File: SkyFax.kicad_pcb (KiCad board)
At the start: 2 copper layers, 50.9 x 101.5 mm, 80 parts, among them J1 RJ11/12, J2 USB_B_Micro, J3 Conn_02x06_Odd_Even, J4 Conn_02x02_Odd_Even, Q1 Q_NPN_BEC, Q2 Q_PNP_BEC, Q3 Q_NPN_BEC, Q4 Q_NPN_BEC, Q5 Q_NPN_BEC, Q6 Q_NPN_EBC, SW2 SW_Push, U1 Si2494-A-FM, U2 Si3018, U3 25LC640AT-E/SN, U4 CP2102N-Axx-xQFN20, X1 ECS-2520MV-xxx-xx

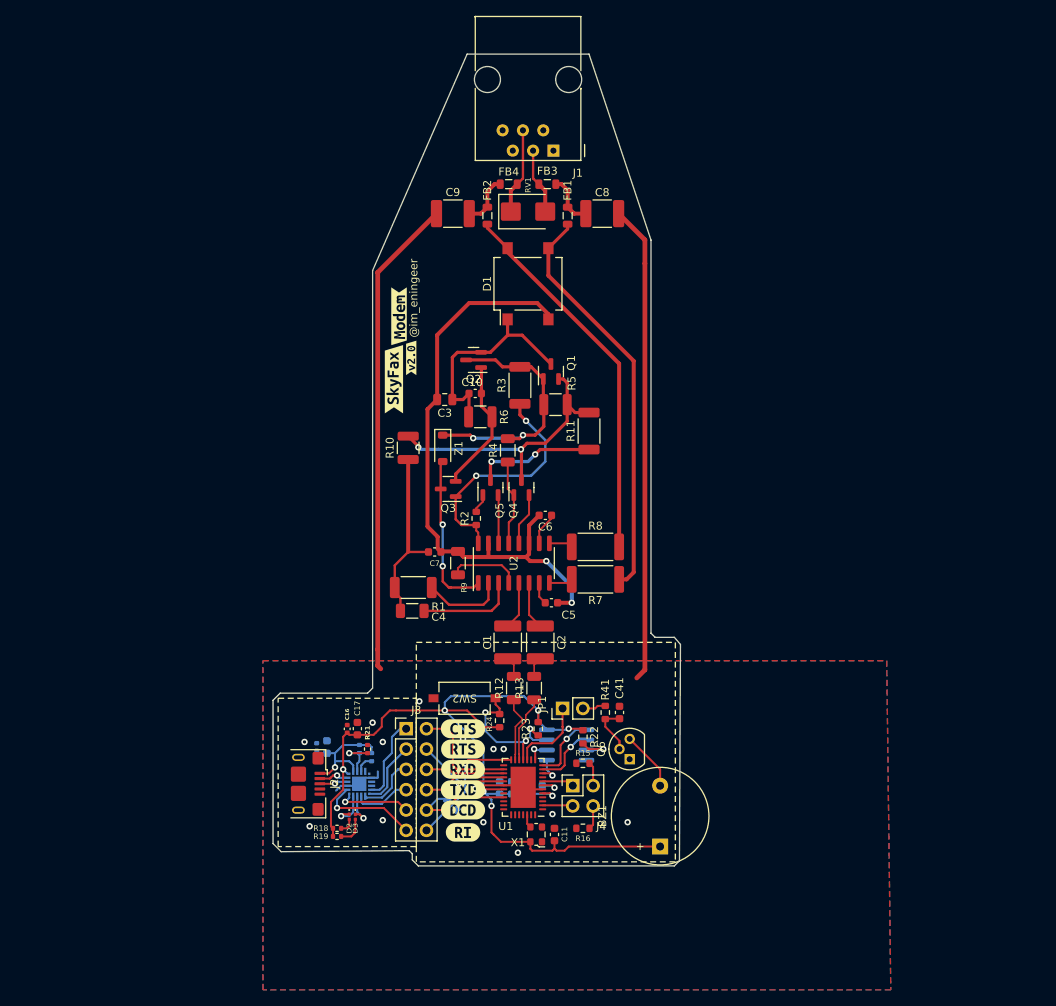
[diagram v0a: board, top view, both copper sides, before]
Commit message: Sent to fab v3.0
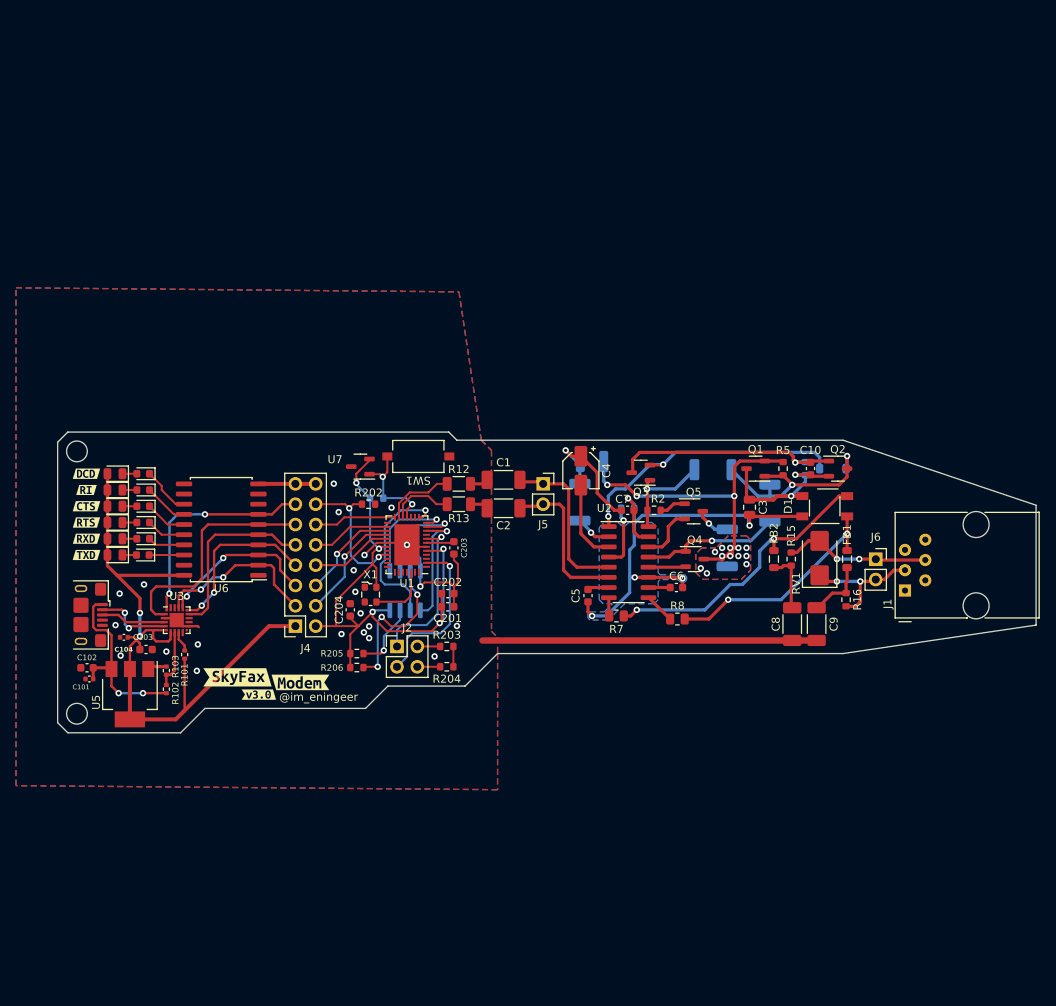
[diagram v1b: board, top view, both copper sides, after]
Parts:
- removed BZ1: Buzzer, Buzzer_Beeper:Buzzer_12x9.5RM7.6
- removed C11, C12, C17, C41, C50, C52: 0.1uF, Capacitor_SMD:C_0603_1608Metric
- removed C13, C16: 4.7uF, Capacitor_SMD:C_0402_1005Metric
- removed C51: 0.22uF, Capacitor_SMD:C_0603_1608Metric
- removed FB3, FB4: FerriteBead_Small, Inductor_SMD:L_0805_2012Metric
- removed JP1: Jumper_2_Open, Connector_PinHeader_2.54mm:PinHeader_1x02_P2.54mm_Vertical
- removed Q6: Q_NPN_EBC, Package_TO_SOT_THT:TO-92
- removed R14, R22, R23, R24: 10k, Resistor_SMD:R_0603_1608Metric
- removed R17: 1k, Resistor_SMD:R_0402_1005Metric
- removed R18, R19: 220, Resistor_SMD:R_0402_1005Metric
- removed R20: 22.1k, Resistor_SMD:R_0402_1005Metric
- removed R21: 47.5k, Resistor_SMD:R_0402_1005Metric
- removed R41: 150, Resistor_SMD:R_0603_1608Metric
- removed SW2: SW_Push, Button_Switch_SMD:SW_Tactile_SPST_NO_Straight_CK_PTS636Sx25SMTRLFS
- removed kibuzzard-64B47980: G***, kibuzzard-64B47980
- removed kibuzzard-64B4798B: G***, kibuzzard-64B4798B
- removed kibuzzard-64B47998: G***, kibuzzard-64B47998
- removed kibuzzard-64B479A1: G***, kibuzzard-64B479A1
- removed kibuzzard-64B479A8: G***, kibuzzard-64B479A8
- removed kibuzzard-64B479C8: G***, kibuzzard-64B479C8
- removed kibuzzard-64DEBF34: G***, kibuzzard-64DEBF34
- added C101: 4.7uF, Capacitor_SMD:C_0402_1005Metric, F.Cu at (47.3, 137.8)
- added C102: 0.1uF, Capacitor_SMD:C_0603_1608Metric, F.Cu at (47.0, 136.4)
- added C103: 4.7uF, Capacitor_SMD:C_0402_1005Metric, F.Cu at (51.6, 132.6)
- added C104: 0.1uF, Capacitor_SMD:C_0603_1608Metric, F.Cu at (54.4, 134.1)
- added C201: 0.1uF, Capacitor_SMD:C_0603_1608Metric, F.Cu at (92.1, 128.8)
- added C202: 0.1uF, Capacitor_SMD:C_0603_1608Metric, F.Cu at (92.1, 127.1)
- added C203: 0.22uF, Capacitor_SMD:C_0603_1608Metric, F.Cu at (92.8, 121.4)
- added C204: 0.1uF, Capacitor_SMD:C_0603_1608Metric, F.Cu at (79.9, 129.2)
- added D4: LED, LED_SMD:LED_0805_2012Metric, F.Cu at (50.5, 118.2)
- added D5: LED, LED_SMD:LED_0805_2012Metric, F.Cu at (50.5, 116.2)
- added D6: LED, LED_SMD:LED_0805_2012Metric, F.Cu at (50.5, 114.2)
- added D7: LED, LED_SMD:LED_0805_2012Metric, F.Cu at (50.5, 112.1)
- added J5: Conn_01x02, Connector_PinSocket_2.54mm:PinSocket_1x02_P2.54mm_Vertical, F.Cu at (104.0, 113.4)
- added J6: Conn_01x02, Connector_PinSocket_2.54mm:PinSocket_1x02_P2.54mm_Vertical, F.Cu at (145.6, 122.8)
- added R101: 1k, Resistor_SMD:R_0402_1005Metric, F.Cu at (59.2, 134.7)
- added R102: 22.1k, Resistor_SMD:R_0402_1005Metric, F.Cu at (56.9, 139.1)
- added R103: 47.5k, Resistor_SMD:R_0402_1005Metric, F.Cu at (56.9, 136.8)
- added R104: 220, LED_SMD:LED_0603_1608Metric, F.Cu at (53.9, 122.3)
- added R105: 220, LED_SMD:LED_0603_1608Metric, F.Cu at (54.0, 120.3)
- added R106: 220, LED_SMD:LED_0603_1608Metric, F.Cu at (54.0, 118.2)
- added R107: 220, LED_SMD:LED_0603_1608Metric, F.Cu at (54.0, 116.2)
- added R108: 220, LED_SMD:LED_0603_1608Metric, F.Cu at (54.0, 114.2)
- added R109: 220, LED_SMD:LED_0603_1608Metric, F.Cu at (54.0, 112.1)
- added R201: 10k, Resistor_SMD:R_0603_1608Metric, B.Cu at (83.2, 115.2)
- added R202: 10k, Resistor_SMD:R_0603_1608Metric, F.Cu at (82.2, 116.0)
- added R203: 10k, Resistor_SMD:R_0603_1608Metric, F.Cu at (91.9, 133.7)
- added R204: 10k, Resistor_SMD:R_0603_1608Metric, F.Cu at (91.9, 136.3)
- added R205: 10k, Resistor_SMD:R_0603_1608Metric, F.Cu at (80.7, 134.6)
- added R206: 10k, Resistor_SMD:R_0603_1608Metric, F.Cu at (80.7, 136.4)
- added SW1: SW_Push, Button_Switch_SMD:SW_Tactile_SPST_NO_Straight_CK_PTS636Sx25SMTRLFS, F.Cu at (88.4, 110.0)
- added U5: AZ1117-3.3, Package_TO_SOT_SMD:SOT-223-3_TabPin2, F.Cu at (52.3, 139.7)
- added U6: 74LCX541, Package_SO:SOIC-20W_7.5x12.8mm_P1.27mm, F.Cu at (63.8, 119.1)
- added U7: DS1818, Package_TO_SOT_SMD:SOT-23-3, F.Cu at (81.1, 111.3)
- added kibuzzard-64F3F98C: G***, kibuzzard-64F3F98C, F.Cu at (68.5, 139.8)
- added kibuzzard-64F3FC0B: G***, kibuzzard-64F3FC0B, F.Cu at (46.9, 122.3)
- added kibuzzard-64F3FC33: G***, kibuzzard-64F3FC33, F.Cu at (46.9, 120.3)
- added kibuzzard-64F3FC43: G***, kibuzzard-64F3FC43, F.Cu at (46.9, 118.2)
- added kibuzzard-64F3FC6A: G***, kibuzzard-64F3FC6A, F.Cu at (46.9, 116.2)
- added kibuzzard-64F3FC7E: G***, kibuzzard-64F3FC7E, F.Cu at (46.9, 114.2)
- added kibuzzard-64F3FC8A: G***, kibuzzard-64F3FC8A, F.Cu at (46.9, 112.1)
- C1, C2, C8, C9: footprint Capacitor_SMD:C_1812_4532Metric -> FaxCam:C_1808
- C4: footprint Capacitor_SMD:C_1206_3216Metric -> Capacitor_SMD:CP_Elec_4x3
- D1: value DF04S -> HDS10M; footprint Diode_SMD:Diode_Bridge_OnSemi_SDIP-4L -> FaxCam:Diodes_Inc_4-SMD
- D2, D3: footprint LED_SMD:LED_0201_0603Metric -> LED_SMD:LED_0805_2012Metric
- J2: value USB_B_Micro -> Conn_02x02_Odd_Even; footprint Connector_USB:USB_Micro-B_Amphenol_10118193-0001LF_Horizontal -> Connector_PinHeader_2.54mm:PinHeader_2x02_P2.54mm_Vertical
- J3: value Conn_02x06_Odd_Even -> USB_B_Micro; footprint Connector_PinHeader_2.54mm:PinHeader_2x06_P2.54mm_Vertical -> Connector_USB:USB_Micro-B_Amphenol_10118193-0001LF_Horizontal
- J4: value Conn_02x02_Odd_Even -> Conn_02x08_Odd_Even; footprint Connector_PinHeader_2.54mm:PinHeader_2x02_P2.54mm_Vertical -> Connector_PinSocket_2.54mm:PinSocket_2x08_P2.54mm_Vertical
- Q1, Q2, Q3, Q4, Q5: footprint Package_TO_SOT_SMD:SOT-23 -> Package_TO_SOT_SMD:SOT-23-3
- R1, R10, R11, R3, Z1: moved to B.Cu
- R15, R16: value 10k -> 0
- R4: footprint Resistor_SMD:R_1206_3216Metric -> Resistor_SMD:R_2010_5025Metric; moved to B.Cu
- R5: footprint Resistor_SMD:R_1210_3225Metric -> Resistor_SMD:R_0603_1608Metric
- R6: footprint Resistor_SMD:R_1210_3225Metric -> Resistor_SMD:R_0603_1608Metric; moved to B.Cu
- R7, R8: footprint Resistor_SMD:R_2512_6332Metric -> Resistor_SMD:R_0805_2012Metric
- R9: footprint Resistor_SMD:R_1206_3216Metric -> Resistor_SMD:R_0603_1608Metric; moved to B.Cu
- U3: value 25LC640AT-E/SN -> CP2102N-Axx-xQFN20; footprint Package_SO:SOIC-8_3.9x4.9mm_P1.27mm -> Package_DFN_QFN:SiliconLabs_QFN-20-1EP_3x3mm_P0.5mm_EP1.8x1.8mm; moved to F.Cu
- U4: value CP2102N-Axx-xQFN20 -> 25LC640AT-E/SN; footprint Package_DFN_QFN:SiliconLabs_QFN-20-1EP_3x3mm_P0.5mm_EP1.8x1.8mm -> Package_SO:SOIC-8_3.9x4.9mm_P1.27mm
- moved J1 70.4 mm to (149.2, 126.7), turned to 90 degrees
- moved C9 68.6 mm to (138.2, 130.9), turned to -90 degrees
- moved RV1 56.6 mm to (138.6, 122.7), turned to 90 degrees
- moved C8 56.5 mm to (135.1, 130.9), turned to -90 degrees
- moved FB2 55.9 mm to (132.8, 122.8), turned to -90 degrees
- moved FB1 55.3 mm to (142.0, 122.8), turned to -90 degrees
- moved U3 51.2 mm to (58.2, 130.4), turned to 0 degrees
- moved Z1 48.8 mm to (140.2, 111.5), turned to 180 degrees
- moved Q2 47.5 mm to (140.8, 111.5), turned to 0 degrees
- moved kibuzzard-64DEBF1B 47.4 mm to (73.7, 138.2), turned to 0 degrees
- moved D1 46.4 mm to (139.2, 116.2)
- moved D3 45.9 mm to (50.5, 120.3), turned to 180 degrees
- moved D2 43.9 mm to (50.5, 122.3), turned to 180 degrees
- moved R16 43.6 mm to (141.9, 127.9), turned to -90 degrees
- moved J3 43.1 mm to (46.2, 129.8), turned to -90 degrees
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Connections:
- net /1_N renamed Net-(C2-Pad2)
- net /1_P renamed Net-(C1-Pad2)
- net /C1_N renamed /SI2494/C2A
- net /C1_P renamed /SI2494/C1A
- net /CLK renamed Net-(U1-CLKIN_XTAL1)
- net Net-(U2-C1B) renamed /SI3018/C1A
- net Net-(U2-C2B) renamed /SI3018/C2A
- D1 pad 2: GND1 -> Net-(D1-Pad2)
- D1 pad 3: Net-(D1-Pad3) -> GND1
- D2 pad 2: Net-(D2-A) -> +3V3
- D3 pad 2: Net-(D3-A) -> +3V3
- FB1 pad 1: Net-(D1-Pad3) -> Net-(D1-Pad4)
- FB1 pad 2: Net-(C8-Pad1) -> Net-(C9-Pad1)
- FB2 pad 1: Net-(D1-Pad4) -> Net-(D1-Pad2)
- FB2 pad 2: Net-(C9-Pad1) -> Net-(C8-Pad1)
- J1 pad 3: /RING -> /SI3018/TIP
- J1 pad 4: /TIP -> /SI3018/RING
- J2 pad 1: VBUS -> /SI2494/SDI
- J2 pad 2: /USB_DM -> Net-(J2-Pin_2)
- J2 pad 3: /USB_DP -> /SI2494/nFSYNC
- J2 pad 4: unconnected-(J2-ID-Pad4) -> Net-(J2-Pin_4)
- J3 pad 1: Net-(J3-Pin_1) -> VBUS
- J3 pad 2: /nCTS -> Net-(J3-D-)
- J3 pad 3: Net-(J3-Pin_3) -> Net-(J3-D+)
- J3 pad 4: /nRTS -> unconnected-(J3-ID-Pad4)
- J3 pad 5: Net-(J3-Pin_5) -> GND
- J3 pad 6: /RXD -> GND
- J4 pad 1: /SDI -> +3V3
- J4 pad 2: Net-(J4-Pin_2) -> +3V3
- J4 pad 3: /nFSYNC -> /USB_Serial/TXD
- J4 pad 4: Net-(J4-Pin_4) -> /SI2494/TXD
- Q3 pad 2: Net-(Q2-B) -> Net-(Q3-E)
- Q3 pad 3: Net-(Q3-E) -> Net-(Q2-B)
- R15 pad 1: Net-(J4-Pin_2) -> Net-(C8-Pad1)
- R15 pad 2: GND -> /SI3018/RING
- R16 pad 1: Net-(J4-Pin_4) -> Net-(C9-Pad1)
- R16 pad 2: GND -> /SI3018/TIP
- R7 pad 1: Net-(D1-Pad3) -> Net-(D1-Pad2)
- RV1 pad 1: /TIP -> /SI3018/TIP
- RV1 pad 2: /RING -> /SI3018/RING
- U1 pad 10: /EESDI -> /SI2494/EESDI
- U1 pad 11: /EESDO -> /SI2494/EESDO
- U1 pad 12: /EECS -> /SI2494/EECS
- U1 pad 13: /EECLK -> /SI2494/EECLK
- U1 pad 15: /AOUT -> unconnected-(U1-AOUT-Pad15)
- U1 pad 16: /RST -> /SI2494/RST
- U1 pad 19: /nRI -> /SI2494/nRI
- U1 pad 2: /nFSYNC -> /SI2494/nFSYNC
- U1 pad 21: /nCTS -> /SI2494/nCTS
- U1 pad 22: /RXD -> /SI2494/RXD
- U1 pad 23: /TXD -> /SI2494/TXD
- U1 pad 24: /nRTS -> /SI2494/nRTS
- U1 pad 28: /nDCD -> /SI2494/nDCD
- U1 pad 35: /nINT -> unconnected-(U1-nINT-Pad35)
- U1 pad 8: /SDI -> /SI2494/SDI
- U3 pad 1: /EECS -> /USB_Serial/DCD
- U3 pad 2: /EESDO -> /USB_Serial/RI
- U3 pad 3: Net-(U3-~{WP}) -> GND
- U3 pad 4: GND -> Net-(J3-D+)
- U3 pad 5: /EESDI -> Net-(J3-D-)
- U3 pad 6: /EECLK -> +3V3
- U3 pad 7: Net-(U3-~{HOLD}) -> +3V3
- U3 pad 8: +3V3 -> Net-(U3-VBUS)
- U4 pad 1: Net-(J3-Pin_9) -> /SI2494/EECS
- U4 pad 2: Net-(J3-Pin_11) -> /SI2494/EESDO
- U4 pad 3: GND -> Net-(U4-~{WP})
- U4 pad 4: /USB_DP -> GND
- U4 pad 5: /USB_DM -> /SI2494/EESDI
- U4 pad 6: +3V3 -> /SI2494/EECLK
- U4 pad 7: VBUS -> Net-(U4-~{HOLD})
- U4 pad 8: Net-(U4-VBUS) -> +3V3
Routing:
- net Net-(D1-Pad3): track 51.1 -> 0.00 mm
- net GND: track 135.4 -> 85.5 mm, vias 14 -> 22
- net +3V3: track 114.0 -> 156.3 mm
- net Net-(D1-Pad2): track 0.00 -> 36.8 mm, vias 0 -> 2
- net /USB_Serial/RI: track 0.00 -> 29.2 mm
- net /USB_Serial/DCD: track 0.00 -> 27.8 mm, vias 0 -> 2
- net /USB_Serial/CTS: track 0.00 -> 22.8 mm
- net /USB_Serial/RTS: track 0.00 -> 21.1 mm, vias 0 -> 2
- net /USB_Serial/TXD: track 0.00 -> 21.0 mm, vias 0 -> 2
- net /SI2494/EECLK: track 0.00 -> 20.9 mm, vias 0 -> 1
- net /SI2494/nFSYNC: track 0.00 -> 20.5 mm, vias 0 -> 1
- net /USB_Serial/RXD: track 0.00 -> 20.0 mm, vias 0 -> 2
- net /SI2494/SDI: track 0.00 -> 19.7 mm, vias 0 -> 1
- net Net-(U4-~{WP}): track 0.00 -> 19.6 mm, vias 0 -> 3
- net /SI3018/RING: track 0.00 -> 18.4 mm, vias 0 -> 2
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- added copper zone on B.Cu, net GND1
- added copper zone on B.Cu, net Net-(Q1-E)
- added copper zone on F.Cu, net Net-(Q1-E)
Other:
- board size 50.9 x 101.5 mm -> 122.3 x 37.6 mm
- board text added: "Intentionally left empty (DRC/ERC will fail here)"
